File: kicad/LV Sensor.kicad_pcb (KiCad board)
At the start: 2 copper layers, 69 parts, among them IC1 MCP2517FDT-H_SL, IC2 L78L05ABUTR, IC3 TLV74133PDBVR, IC4 TLV74125PDBVR, J1 Screw_Terminal_01x02, J16 USB_B_Micro, J2 Screw_Terminal_01x02, J3 Screw_Terminal_01x02, J4 Screw_Terminal_01x02, J5 Screw_Terminal_01x02, J6 43650-0401, SW1 SW_Push, U0 AP63205WU-7, U10 MCP3204-CI/P, U2 XMSM0C1104SPW20R, U3 FT231XS-R, U6 DSC1001DL5-020.0000T, U7 ADS114S06BIPBSR, U8 LM2662MX/NOPB, U9 ATA6561-GAQW-N

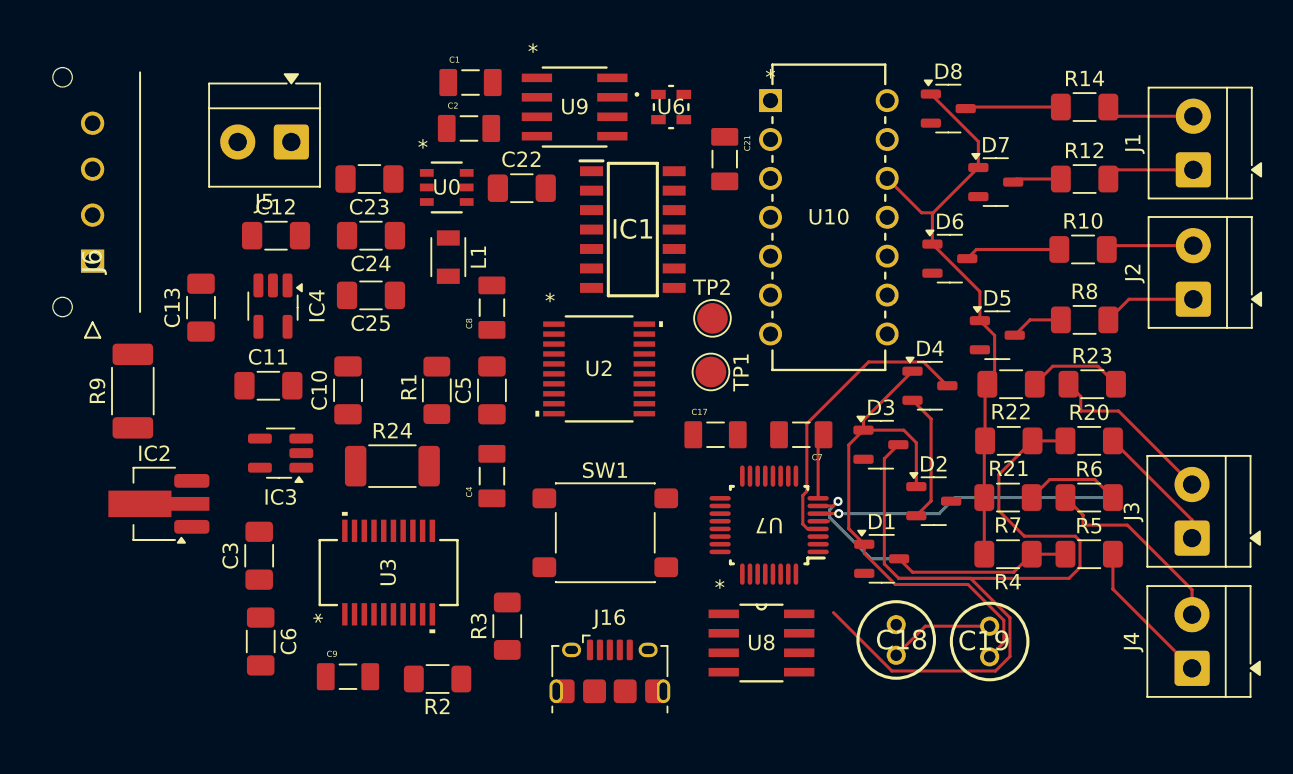
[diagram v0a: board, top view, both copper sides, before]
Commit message: finalized changes
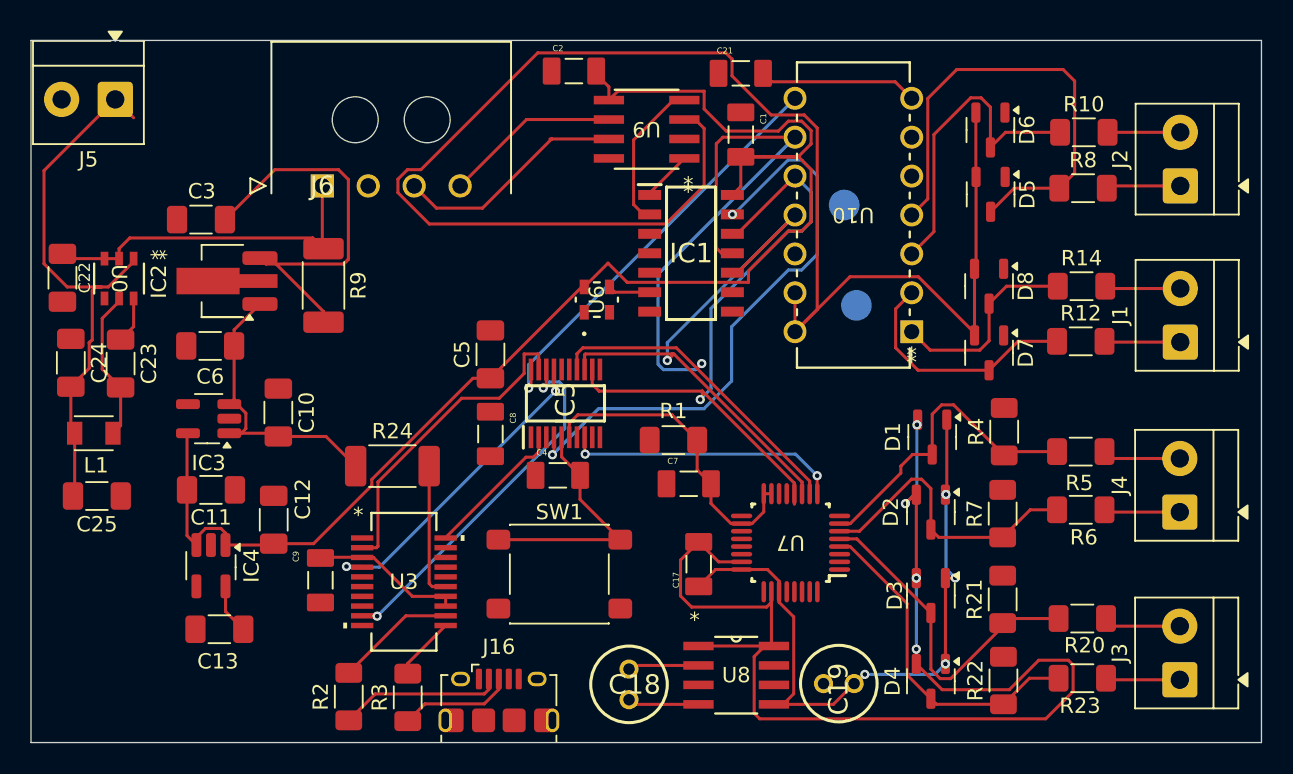
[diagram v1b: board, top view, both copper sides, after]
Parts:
- removed U2: XMSM0C1104SPW20R, LV-Sensor-Footprints-Lib:TSSOP20_PW_TEX
- added IC5: MSPM0C1104SDGS20R, LV-Sensor-Footprints-Lib:SOP50P490X110-20N, F.Cu at (184.2, 75.8)
- J6: footprint ADC2_AND_4:43650-04YY_151617 -> LV-Sensor-Footprints-Lib:43650-04_00,01,02_
- TP1, TP2: moved to B.Cu
- moved C22 30.6 mm to (151.3, 67.7), turned to -90 degrees
- moved L1 25.8 mm to (153.4, 77.8), turned to 0 degrees
- moved C3 22.3 mm to (160.4, 63.9), turned to 0 degrees
- moved U0 22.2 mm to (155.1, 67.7), turned to -90 degrees
- moved C25 22.2 mm to (153.6, 81.9)
- moved C24 21.3 mm to (151.9, 73.2), turned to -90 degrees
- moved C13 21.0 mm to (161.6, 90.6), turned to 180 degrees
- moved C23 20.2 mm to (155.2, 73.2), turned to -90 degrees
- moved C6 19.6 mm to (161.0, 72.1), turned to 0 degrees
- moved R22 19.4 mm to (212.8, 94.0), turned to 90 degrees
- moved D4 19.3 mm to (208.1, 94.0), turned to -90 degrees
- moved R23 19.2 mm to (217.9, 93.8), turned to 180 degrees
- moved C12 18.6 mm to (165.2, 83.5), turned to 90 degrees
- moved C1 18.0 mm to (195.7, 58.3), turned to -90 degrees
- moved C18 17.7 mm to (188.3, 94.2)
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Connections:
- C18 pad 2: GND -> Net-(U8-C1-)
- IC1 pad 13: Net-(IC1-NCS) -> CS_CAN
- R20 pad 2: Net-(J3-Pin_1) -> Net-(J3-Pin_2)
- R23 pad 1: Net-(J3-Pin_2) -> Net-(J3-Pin_1)
- R5 pad 2: Net-(J4-Pin_1) -> Net-(J4-Pin_2)
- R6 pad 1: Net-(J4-Pin_2) -> Net-(J4-Pin_1)
- U10 pad 8: Net-(U10-CS/SHDN) -> CS_ADC4
- U3 pad 2: /UART0_RTS -> UART0_RTS
- U3 pad 20: /UART0_TX -> UART0_TX
- U3 pad 4: /UART0_RX -> UART0_RX
- U3 pad 9: /UART0_CTS -> UART0_CTS
- U7 pad 9: Net-(U2-PA2) -> CS_ADC8
- U8 pad 4: GND -> Net-(U8-C1-)
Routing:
- net +5V: track 0.00 -> 127.5 mm
- net +3V3: track 0.00 -> 116.3 mm
- net +2V5: track 8.44 -> 84.3 mm, vias 0 -> 4
- net Net-(IC1-SDI): track 0.00 -> 56.9 mm, vias 0 -> 1
- net GND: track 49.6 -> 0.00 mm
- net Net-(IC1-SDO): track 0.00 -> 43.7 mm, vias 0 -> 1
- net Net-(D3-COM): track 62.1 -> 22.0 mm
- net Net-(IC1-SCK): track 0.00 -> 38.6 mm, vias 0 -> 1
- net CS_CAN: track 0.00 -> 38.6 mm, vias 0 -> 2
- net /5V out: track 0.00 -> 36.6 mm
- net Net-(D5-COM): track 3.43 -> 31.3 mm
- net Net-(IC2-VIN): track 0.00 -> 27.6 mm
- net CS_ADC4: track 0.00 -> 27.4 mm, vias 0 -> 1
- net UART0_CTS: track 0.00 -> 24.0 mm, vias 0 -> 2
- net +12V: track 0.00 -> 22.5 mm
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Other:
- board outline added: 80.3 x 45.9 mm
